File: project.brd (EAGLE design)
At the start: 48.3 x 107.9 mm, 47 parts, among them IC1 ON MC34063A, IC2 78L15Z, J2 AUDIO_JACK_3.5MM_KIT, J3 AUDIO_JACK_3.5MM_KIT, J4 AUDIO_JACK_3.5MM_KIT, U1 TL071, U2 TL071, X1 CONRAD_736880-49, X2 CONRAD_736880-49

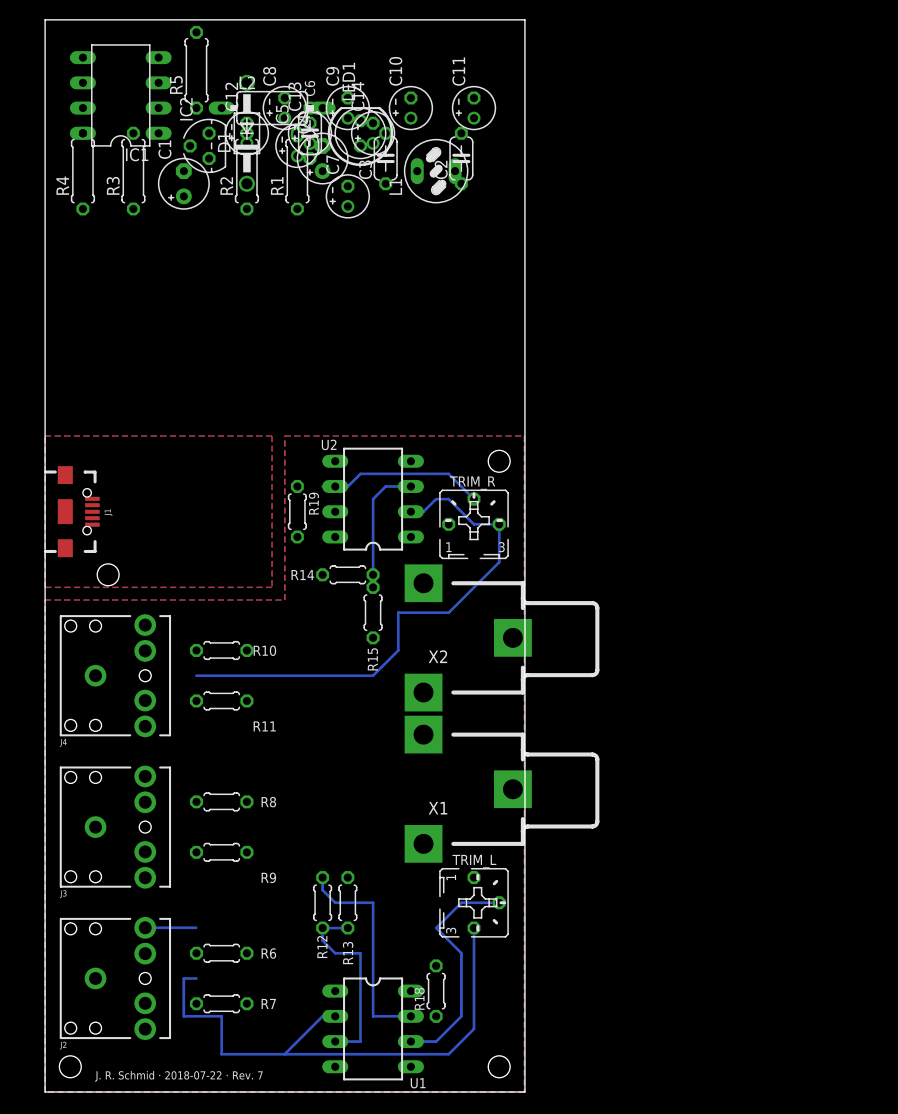
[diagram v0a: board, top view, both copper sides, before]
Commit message: Re-doing the PCB.
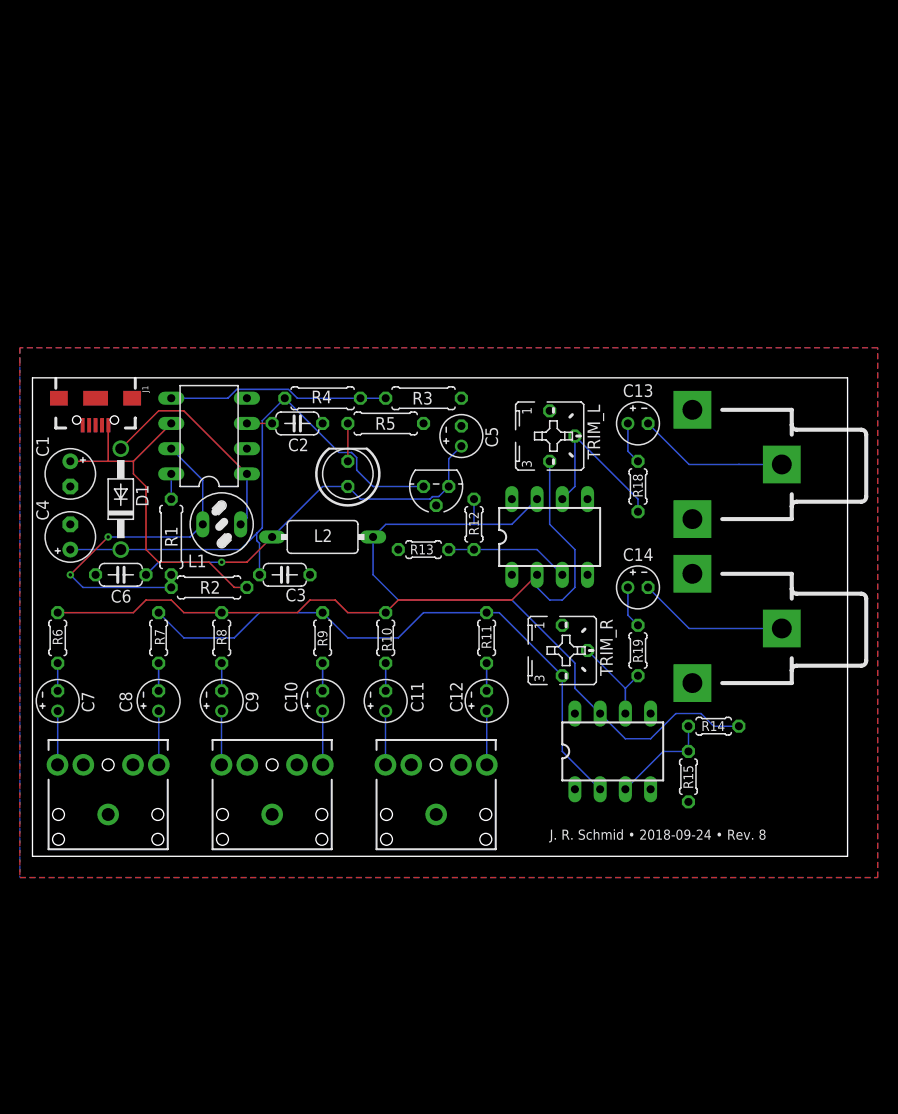
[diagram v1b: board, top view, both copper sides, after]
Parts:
- moved C12 62.0 mm to (45.7, 40.6)
- moved C8 61.0 mm to (12.7, 40.6)
- moved C9 61.0 mm to (19.1, 40.6)
- moved C10 60.3 mm to (29.2, 40.6)
- moved C11 60.3 mm to (35.6, 40.6)
- moved C7 58.6 mm to (2.54, 40.6)
- moved R18 54.7 mm to (61.0, 62.2)
- moved C14 52.9 mm to (61.0, 52.1), turned to 0 degrees
- moved U1 52.6 mm to (52.1, 57.1), turned to 0 degrees
- moved C6 48.4 mm to (8.89, 53.3), turned to 0 degrees
- moved TRIM_L 47.6 mm to (52.1, 67.3)
- moved C4 45.8 mm to (3.81, 57.1)
- moved C13 44.1 mm to (61.0, 68.6), turned to 0 degrees
- moved L2 43.5 mm to (29.2, 57.1)
- moved C3 43.1 mm to (25.4, 53.3), turned to 180 degrees
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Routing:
- net N$23: track 0.00 -> 56.9 mm
- net VCC: track 22.1 -> 71.2 mm
- net N$22: track 0.00 -> 39.8 mm, vias 0 -> 1
- net N$29: track 0.00 -> 36.5 mm
- net N$31: track 0.00 -> 36.3 mm, vias 0 -> 2
- net N$28: track 0.00 -> 22.3 mm
- net N$11: track 0.00 -> 22.3 mm
- net N$12: track 56.0 -> 71.8 mm
- net N$3: track 0.00 -> 15.2 mm
- net N$1: track 0.00 -> 15.2 mm
- net N$33: track 51.7 -> 60.5 mm
- net N$9: track 19.6 -> 12.5 mm
- net N$24: track 16.8 -> 9.72 mm
- net N$5: track 23.5 -> 17.1 mm
- net N$20: track 0.00 -> 5.42 mm
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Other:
- board size 48.3 x 107.9 mm -> 82.1 x 48.2 mm
- board text added: "J. R. Schmid • 2018-09-24 • Rev. 8"
- board text removed: "3-WAY HI-FI DISTRIBUTOR"
- board text removed: "J. R. Schmid · 2018-07-22 · Rev. 7"
- board text removed: "The Three Musketeers"
